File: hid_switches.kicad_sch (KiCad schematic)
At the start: 17 parts, among them SW1 DX0, SW10 DX9, SW11 DX10, SW12 DX11, SW2 DX1, SW3 DX2, SW4 DX3, SW5 DX4, SW6 DX5, SW7 DX6, SW8 DX7, SW9 DX8, U11 74LS125, U12 74LS125, U13 74LS125

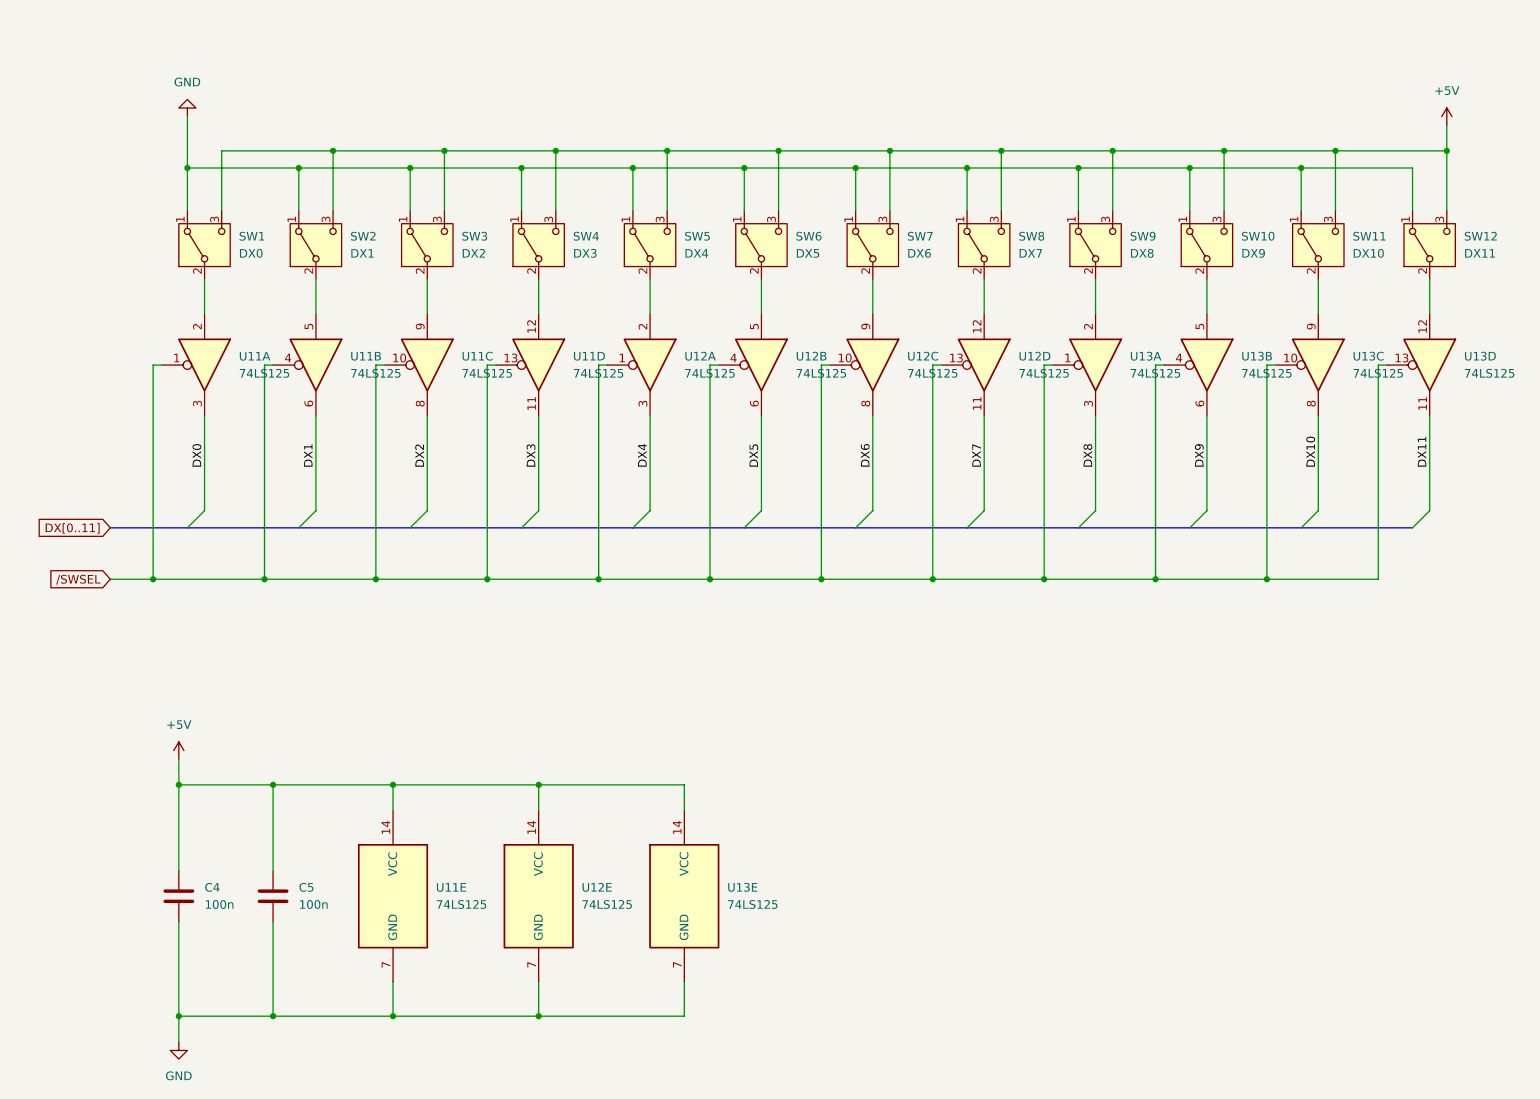
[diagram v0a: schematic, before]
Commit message: HID board finalizing
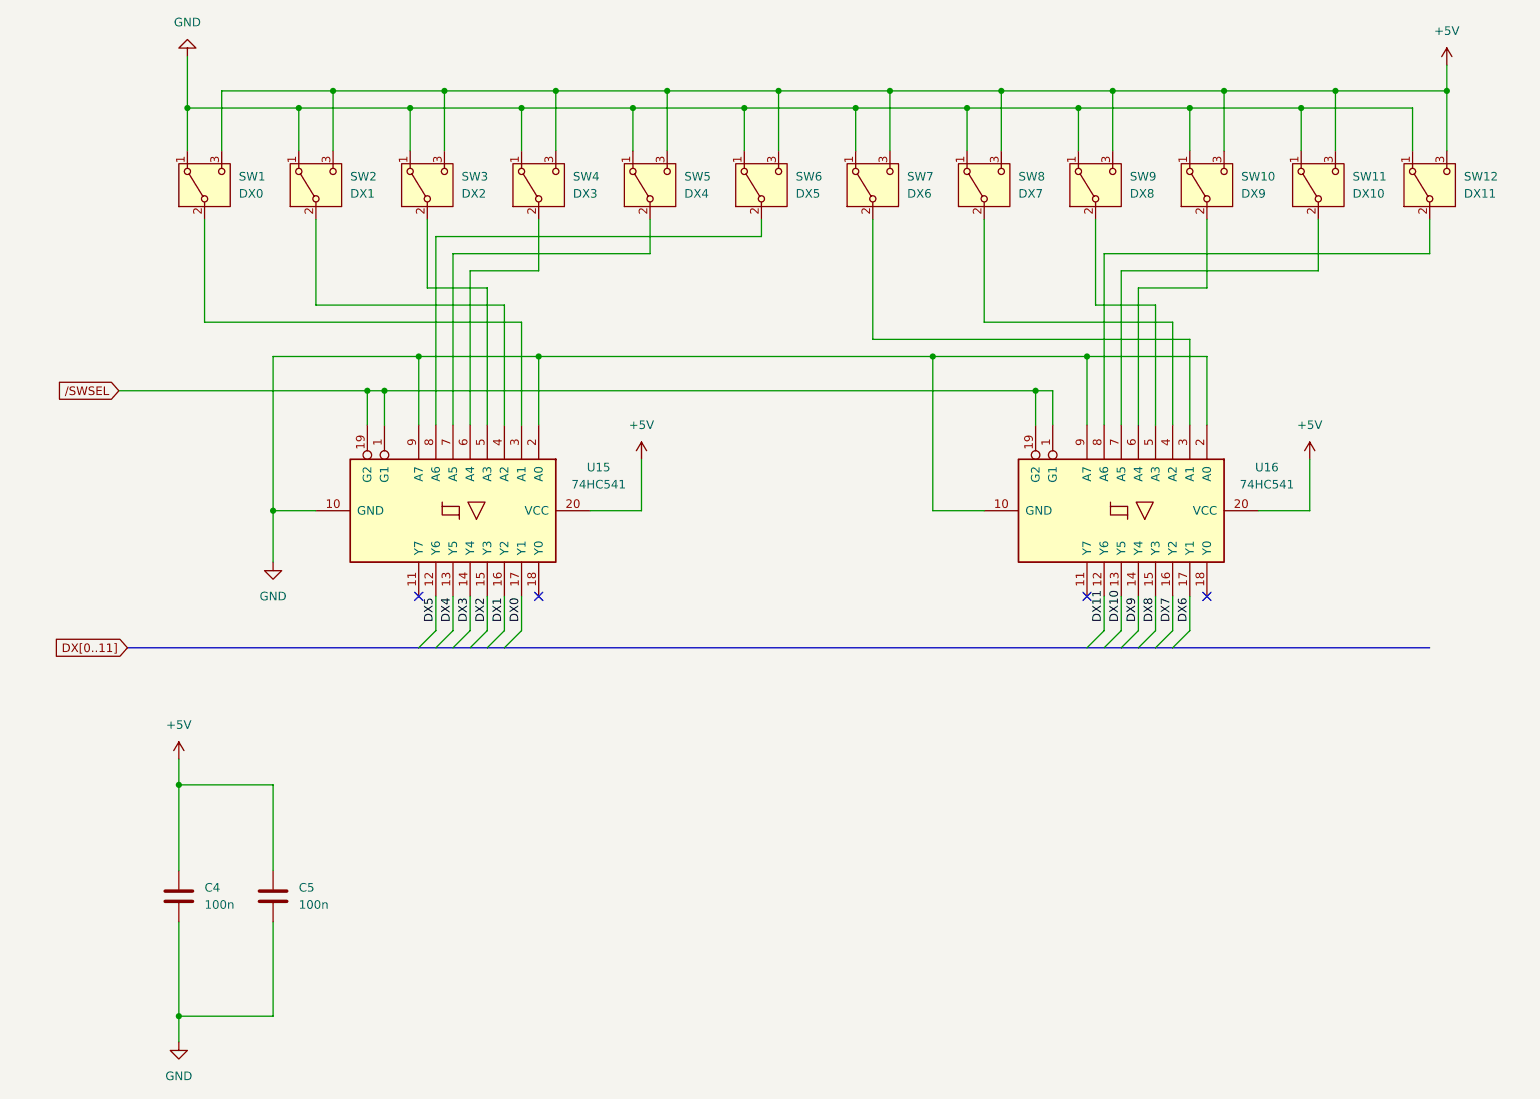
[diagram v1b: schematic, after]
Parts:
- removed U11, U12, U13: 74LS125, Package_SO:SO-14_3.9x8.65mm_P1.27mm, symbol 74xx:74LS125
- added U15, U16: 74HC541, Package_SO:SO-20_12.8x7.5mm_P1.27mm, symbol 74xx:74HCT541
- C4, C5: footprint Capacitor_THT:C_Disc_D3.8mm_W2.6mm_P2.50mm -> Capacitor_SMD:C_0805_2012Metric_Pad1.18x1.45mm_HandSolder
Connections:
- net +5V: now also U15.20 (VCC), U16.20 (VCC)
- net /SWSEL: now also U15.1 (G1), U15.19 (G2), U16.1 (G1), U16.19 (G2)
- net DX0: now also U15.17 (Y1)
- net DX1: now also U15.16 (Y2)
- net DX10: now also U16.13 (Y5)
- net DX11: now also U16.12 (Y6)
- net DX2: now also U15.15 (Y3)
- net DX3: now also U15.14 (Y4)
- net DX4: now also U15.13 (Y5)
- net DX5: now also U15.12 (Y6)
- net DX6: now also U16.17 (Y1)
- net DX7: now also U16.16 (Y2)
- net DX8: now also U16.15 (Y3)
- net DX9: now also U16.14 (Y4)
- net GND: now also U15.10 (GND), U15.2 (A0), U15.9 (A7), U16.10 (GND), U16.2 (A0), U16.9 (A7)
- net at SW4.2 (B): now also U15.6 (A4)
- net at SW8.2 (B): now also U16.4 (A2)
- net at SW9.2 (B): now also U16.5 (A3)
- net at SW6.2 (B): now also U15.8 (A6)
- net at SW11.2 (B): now also U16.7 (A5)
- net at SW10.2 (B): now also U16.6 (A4)
- net at SW12.2 (B): now also U16.8 (A6)
- net at SW2.2 (B): now also U15.4 (A2)
- net at SW1.2 (B): now also U15.3 (A1)
- net at SW3.2 (B): now also U15.5 (A3)
- net at SW7.2 (B): now also U16.3 (A1)
- net at SW5.2 (B): now also U15.7 (A5)
- no-connect marks 0 -> 4
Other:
- moved on the sheet: SW1, SW10, SW11, SW12, SW2, SW3, SW4, SW5, SW6, SW7, SW8, SW9
